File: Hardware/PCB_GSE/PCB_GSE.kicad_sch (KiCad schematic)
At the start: 0 parts

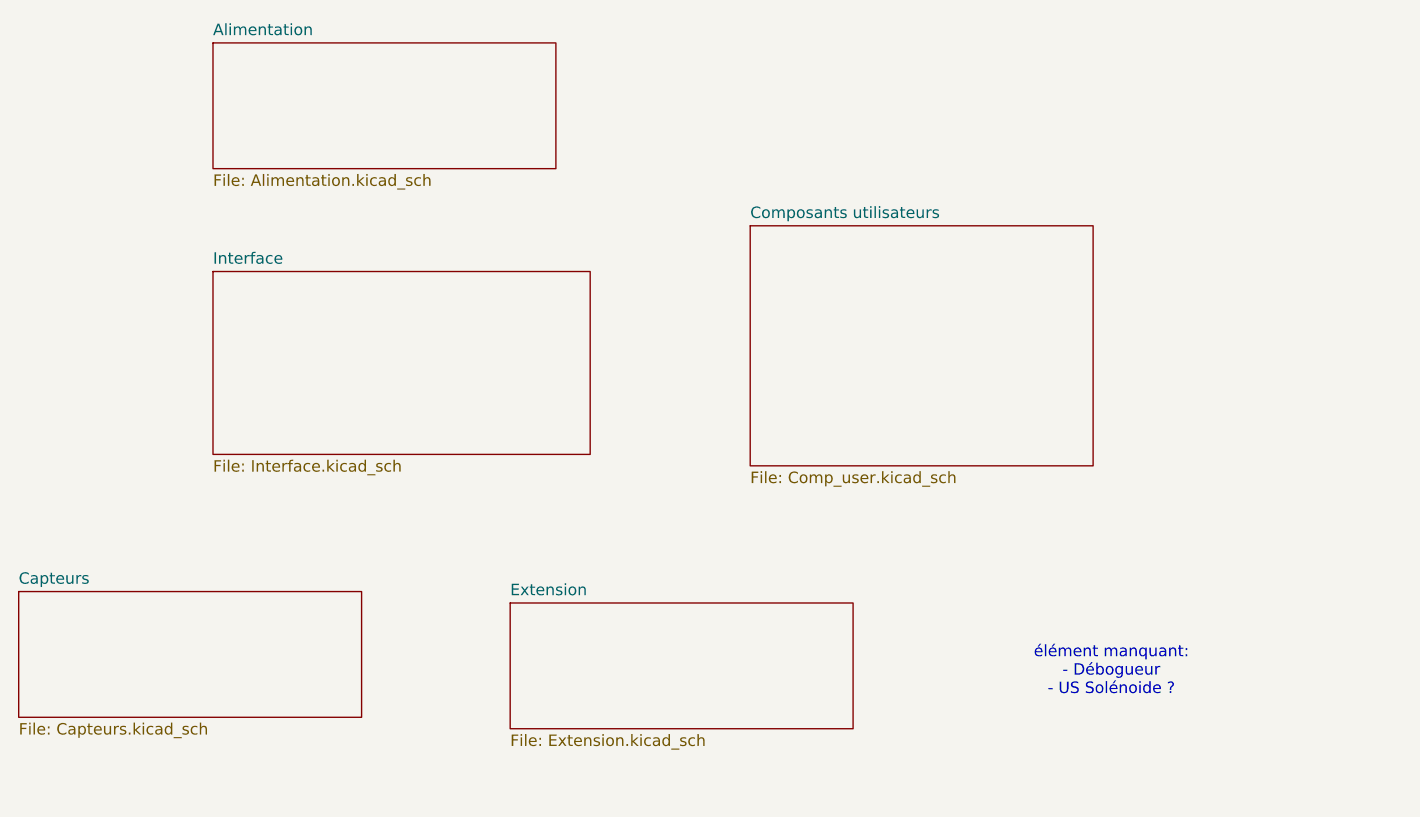
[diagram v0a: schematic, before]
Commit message: un peux d'avancement (brouillon)
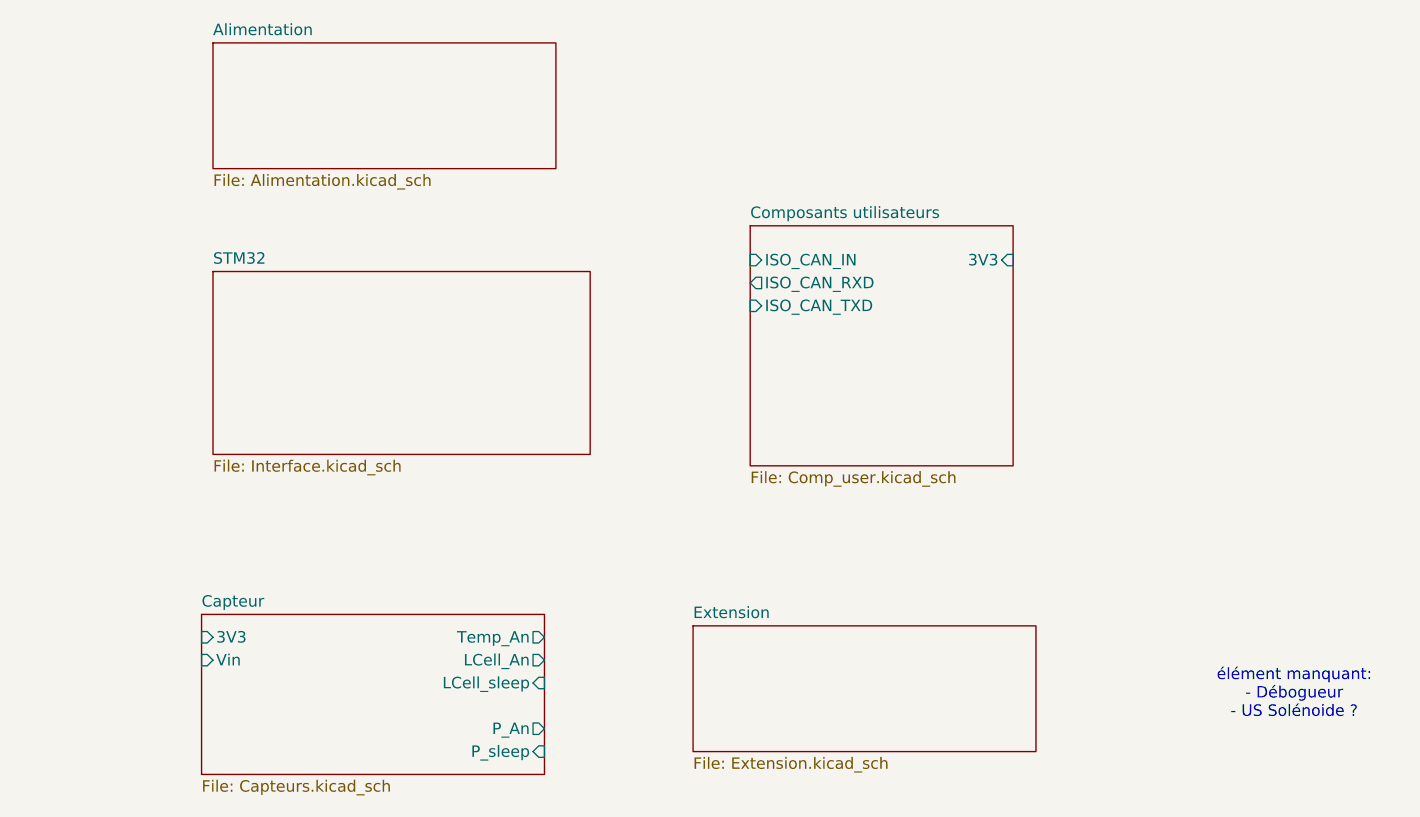
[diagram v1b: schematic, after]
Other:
- sheet Capteurs renamed Capteur
- sheet Interface renamed STM32
- sheet Capteur ports: added 3V3, LCell_An, LCell_sleep, P_An, P_sleep, Temp_An, Vin; removed none
- sheet Composants utilisateurs ports: added 3V3, ISO_CAN_IN, ISO_CAN_RXD, ISO_CAN_TXD; removed none
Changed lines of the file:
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@@
 	(text "élément manquant:\n- Débogueur\n- US Solénoide ?"
 		(exclude_from_sim no)
-		(at 140.462 111.76 0)
+		(at 160.782 114.3 0)
 		(effects
 			(font
@@
 	)
 	(sheet
-		(at 73.66 104.14)
+		(at 93.98 106.68)
 		(size 38.1 13.97)
 		(exclude_from_sim no)
@@
 		)
 		(property "Sheetname" "Extension"
-			(at 73.66 103.4284 0)
+			(at 93.98 105.9684 0)
 			(effects
 				(font
@@
 		)
 		(property "Sheetfile" "Extension.kicad_sch"
-			(at 73.66 118.6946 0)
+			(at 93.98 121.2346 0)
 			(effects
 				(font
@@
 	)
 	(sheet
-		(at 19.05 102.87)
-		(size 38.1 13.97)
-		(exclude_from_sim no)
-		(in_bom yes)
-		(on_board yes)
-		(dnp no)
-		(fields_autoplaced yes)
-		(stroke
-			(width 0.1524)
-			(type solid)
-		)
-		(fill
-			(color 0 0 0 0.0000)
-		)
-		(property "Sheetname" "Capteurs"
-			(at 19.05 102.1584 0)
+		(at 39.37 105.41)
+		(size 38.1 17.78)
+		(exclude_from_sim no)
+		(in_bom yes)
+		(on_board yes)
+		(dnp no)
+		(fields_autoplaced yes)
+		(stroke
+			(width 0.1524)
+			(type solid)
+		)
+		(fill
+			(color 0 0 0 0.0000)
+		)
+		(property "Sheetname" "Capteur"
+			(at 39.37 104.6984 0)
 			(effects
 				(font
@@
 		)
 		(property "Sheetfile" "Capteurs.kicad_sch"
-			(at 19.05 117.4246 0)
-			(effects
-				(font
-					(size 1.27 1.27)
-				)
-				(justify left top)
+			(at 39.37 123.7746 0)
+			(effects
+				(font
+					(size 1.27 1.27)
+				)
+				(justify left top)
+			)
+		)
+		(pin "LCell_An" output
+			(at 77.47 110.49 0)
+			(effects
+				(font
+					(size 1.27 1.27)
+				)
+				(justify right)
+			)
+		)
+		(pin "LCell_sleep" input
+			(at 77.47 113.03 0)
+			(effects
+				(font
+					(size 1.27 1.27)
+				)
+				(justify right)
+			)
+		)
+		(pin "P_An" output
+			(at 77.47 118.11 0)
+			(effects
+				(font
+					(size 1.27 1.27)
+				)
+				(justify right)
+			)
+		)
+		(pin "P_sleep" input
+			(at 77.47 120.65 0)
+			(effects
+				(font
+					(size 1.27 1.27)
+				)
+				(justify right)
+			)
+		)
+		(pin "Temp_An" output
+			(at 77.47 107.95 0)
+			(effects
+				(font
+					(size 1.27 1.27)
+				)
+				(justify right)
+			)
+		)
+		(pin "Vin" input
+			(at 39.37 110.49 180)
+			(effects
+				(font
+					(size 1.27 1.27)
+				)
+				(justify left)
+			)
+		)
+		(pin "3V3" input
+			(at 39.37 107.95 180)
+			(effects
+				(font
+					(size 1.27 1.27)
+				)
+				(justify left)
 			)
 		)
@@
 	(sheet
 		(at 100.33 62.23)
-		(size 38.1 26.67)
+		(size 29.21 26.67)
 		(exclude_from_sim no)
 		(in_bom yes)
@@
 			)
 		)
+		(pin "ISO_CAN_IN" input
+			(at 100.33 66.04 180)
+			(effects
+				(font
+					(size 1.27 1.27)
+				)
+				(justify left)
+			)
+		)
+		(pin "ISO_CAN_RXD" output
+			(at 100.33 68.58 180)
+			(effects
+				(font
+					(size 1.27 1.27)
+				)
+				(justify left)
+			)
+		)
+		(pin "ISO_CAN_TXD" input
+			(at 100.33 71.12 180)
+			(effects
+				(font
+					(size 1.27 1.27)
+				)
+				(justify left)
+			)
+		)
+		(pin "3V3" input
+			(at 129.54 66.04 0)
+			(effects
+				(font
+					(size 1.27 1.27)
+				)
+				(justify right)
+			)
+		)
 		(instances
 			(project "PCB_GSE"
@@
 			(color 0 0 0 0.0000)
 		)
-		(property "Sheetname" "Interface"
+		(property "Sheetname" "STM32"
 			(at 40.64 66.5984 0)
 			(effects
